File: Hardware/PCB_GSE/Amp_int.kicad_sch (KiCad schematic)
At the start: 1 part, among them U1 INA125UA/2K5

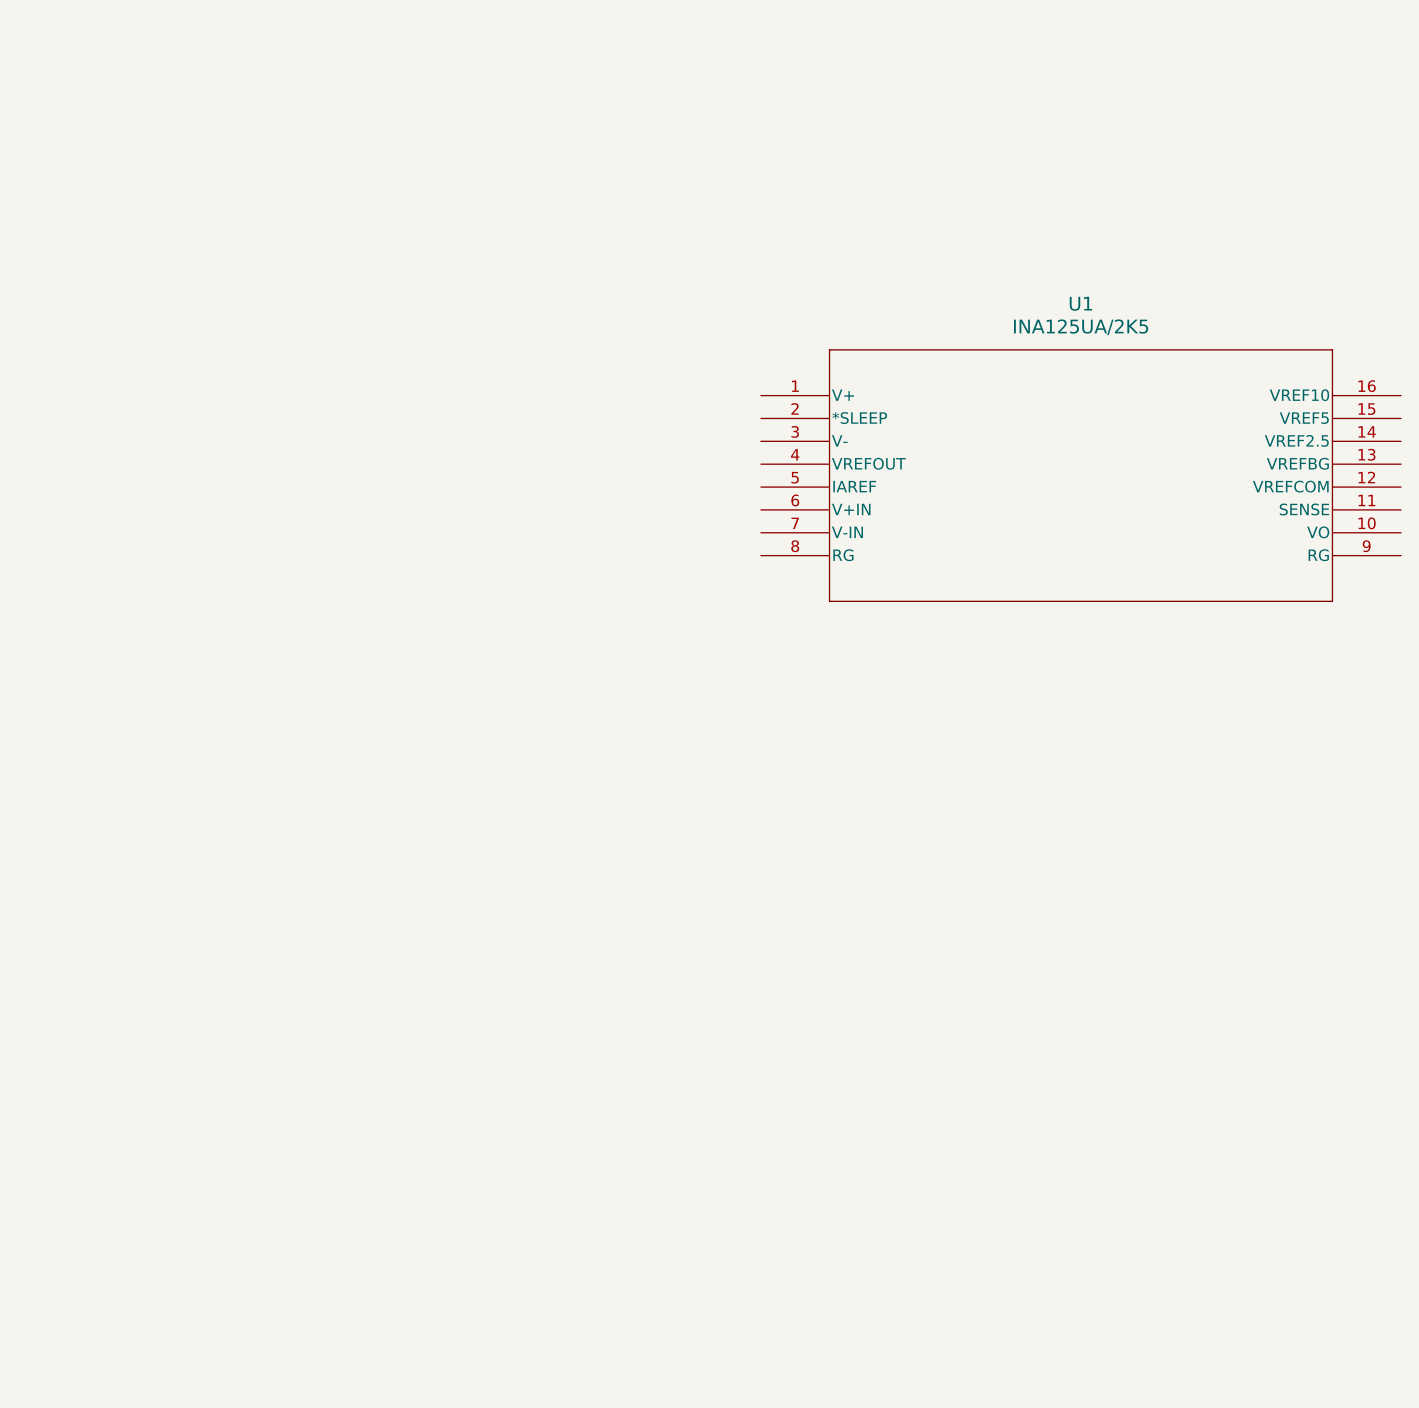
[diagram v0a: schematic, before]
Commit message: un peux d'avancement (brouillon)
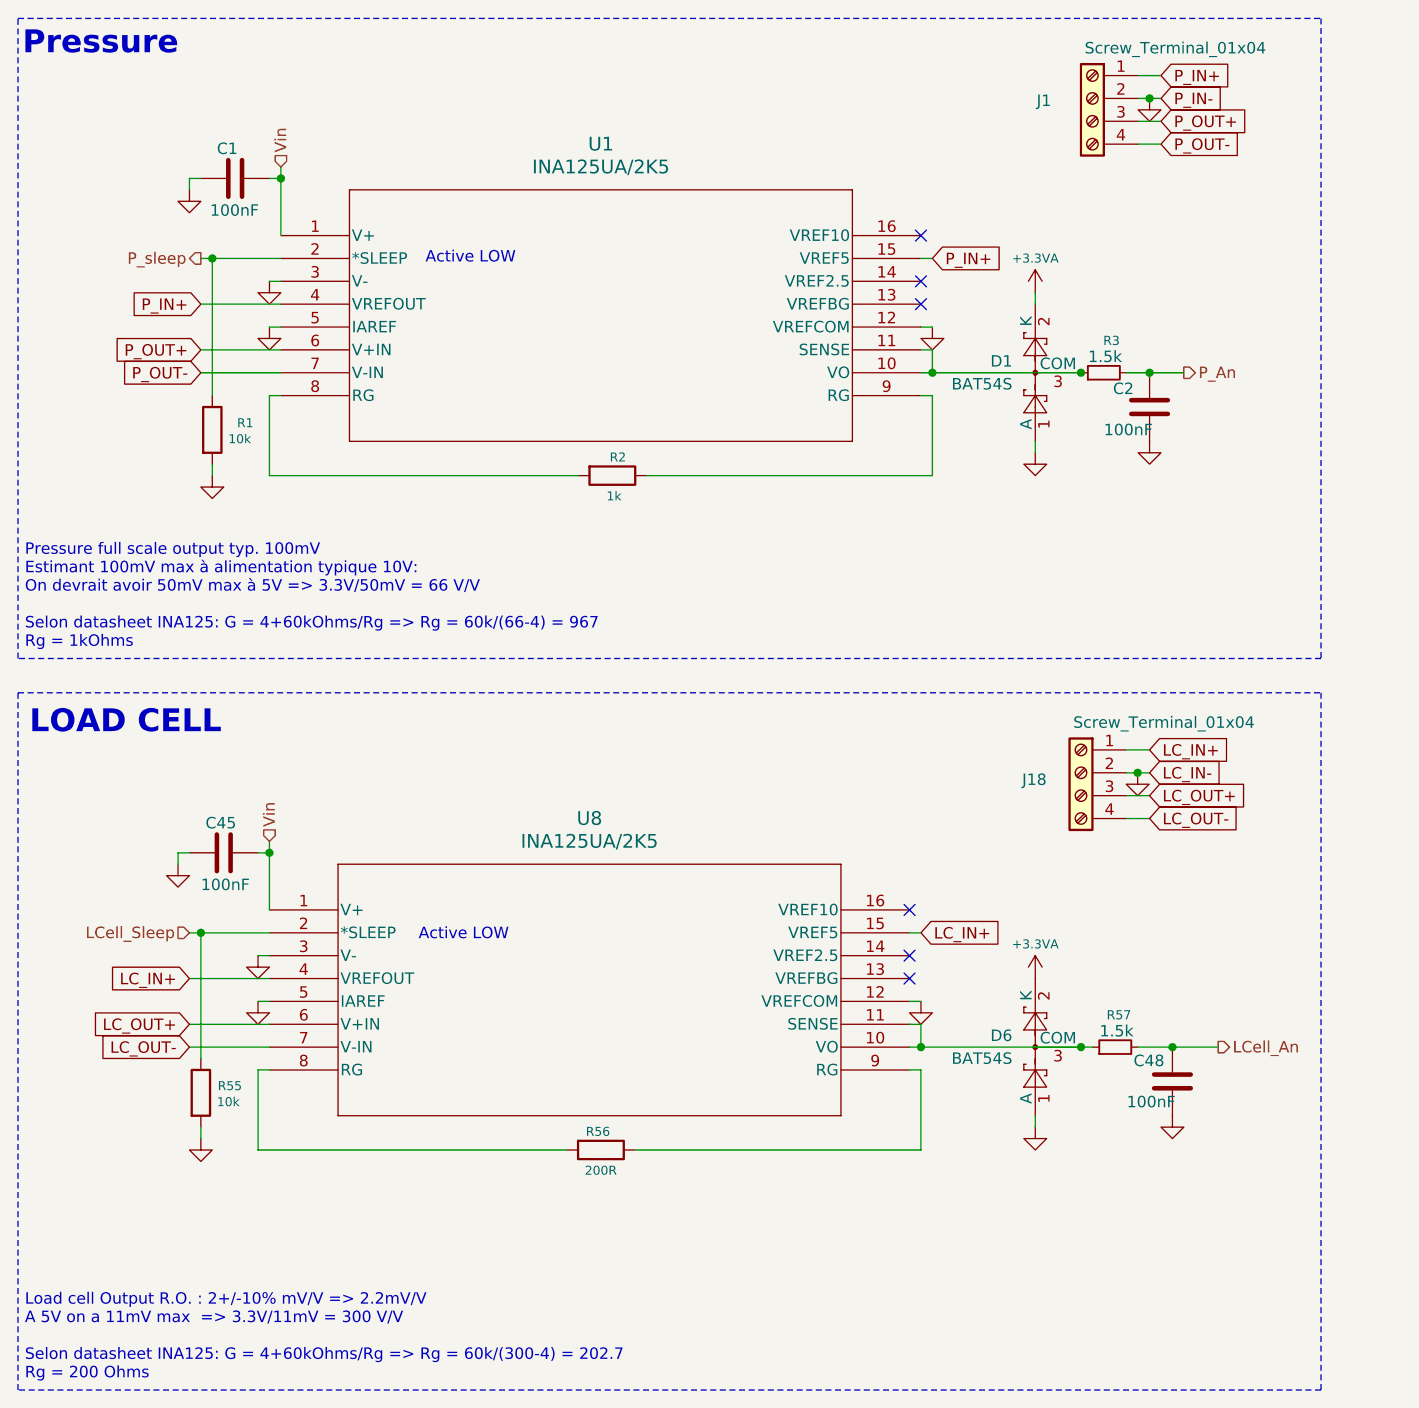
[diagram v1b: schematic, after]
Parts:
- removed U1: INA125UA/2K5, pcb_moteur:D16-L, symbol PCB_GSE:INA125UA_2K5
- added C1, C2, C45, C48: 100nF, Capacitor_SMD:C_0805_2012Metric, symbol Device:C
- added D1, D6: BAT54S, Package_TO_SOT_SMD:SOT-23, symbol Diode:BAT54S
- added J1, J18: Screw_Terminal_01x04, pcb_moteur:CONN_OSTVN04A150_OST, symbol Connector:Screw_Terminal_01x04
- added R1, R55: 10k, Resistor_SMD:R_0805_2012Metric, symbol Device:R
- added R2: 1k, Resistor_SMD:R_0805_2012Metric, symbol Device:R
- added R3, R57: 1.5k, Resistor_SMD:R_0805_2012Metric, symbol Device:R_Small
- added R56: 200R, Resistor_SMD:R_0805_2012Metric, symbol Device:R
- added U1, U8: INA125UA/2K5, pcb_moteur:D16-L, symbol pcb_moteur:INA125UA_2K5
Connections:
- new net: D6.3 (COM), R57.1, U8.10 (VO), U8.11 (SENSE)
- new net: R56.2, U8.8 (RG)
- new net: R56.1, U8.9 (RG)
- new net: D1.3 (COM), R3.1, U1.10 (VO), U1.11 (SENSE)
- new net: R2.1, U1.9 (RG)
- new net: R2.2, U1.8 (RG)
- new net +3.3VA: D1.2 (K), D6.2 (K)
- new net GND: C1.2, C2.2, C45.2, C48.2, D1.1 (A), D6.1 (A), J1.2 (Pin_2), J18.2 (Pin_2), R1.2, R55.2, U1.12 (VREFCOM), U1.3 (V-), U1.5 (IAREF), U8.12 (VREFCOM), U8.3 (V-), U8.5 (IAREF)
- new net LC_IN+: J18.1 (Pin_1), U8.15 (VREF5), U8.4 (VREFOUT)
- new net LC_OUT+: J18.3 (Pin_3), U8.6 (V+IN)
- new net LC_OUT-: J18.4 (Pin_4), U8.7 (V-IN)
- new net LCell_An: C48.1, R57.2
- new net LCell_Sleep: R55.1, U8.2 (*SLEEP)
- new net P_An: C2.1, R3.2
- new net P_IN+: J1.1 (Pin_1), U1.15 (VREF5), U1.4 (VREFOUT)
- new net P_OUT+: J1.3 (Pin_3), U1.6 (V+IN)
- new net P_OUT-: J1.4 (Pin_4), U1.7 (V-IN)
- new net P_sleep: R1.1, U1.2 (*SLEEP)
- new net Vin: C1.1, C45.1, U1.1 (V+), U8.1 (V+)
- no-connect marks 0 -> 6
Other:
- note added: "Active LOW"
- note added: "LOAD CELL"
- note added: "Load cell Output R.O. : 2+/-10% mV/V => 2.2mV/V A 5V on a 11mV max => 3.3V/11mV = 300 V/V Selon datasheet INA125: G = 4+60kOhms/Rg => Rg = 60k/(300-4) = 202.7 Rg = 200 Ohms"
- note added: "Pressure"
- note added: "Pressure full scale output typ. 100mV Estimant 100mV max à alimentation typique 10V: On devrait avoir 50mV max à 5V => 3.3V/50mV = 66 V/V Selon datasheet INA125: G = 4+60kOhms/Rg => Rg = 60k/(66-4) = 967 Rg = 1kOhms"
